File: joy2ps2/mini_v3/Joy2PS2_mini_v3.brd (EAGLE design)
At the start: 25.4 x 47 mm, 8 parts, among them IC1 ATMEGA168PROUND, Q1 BS170

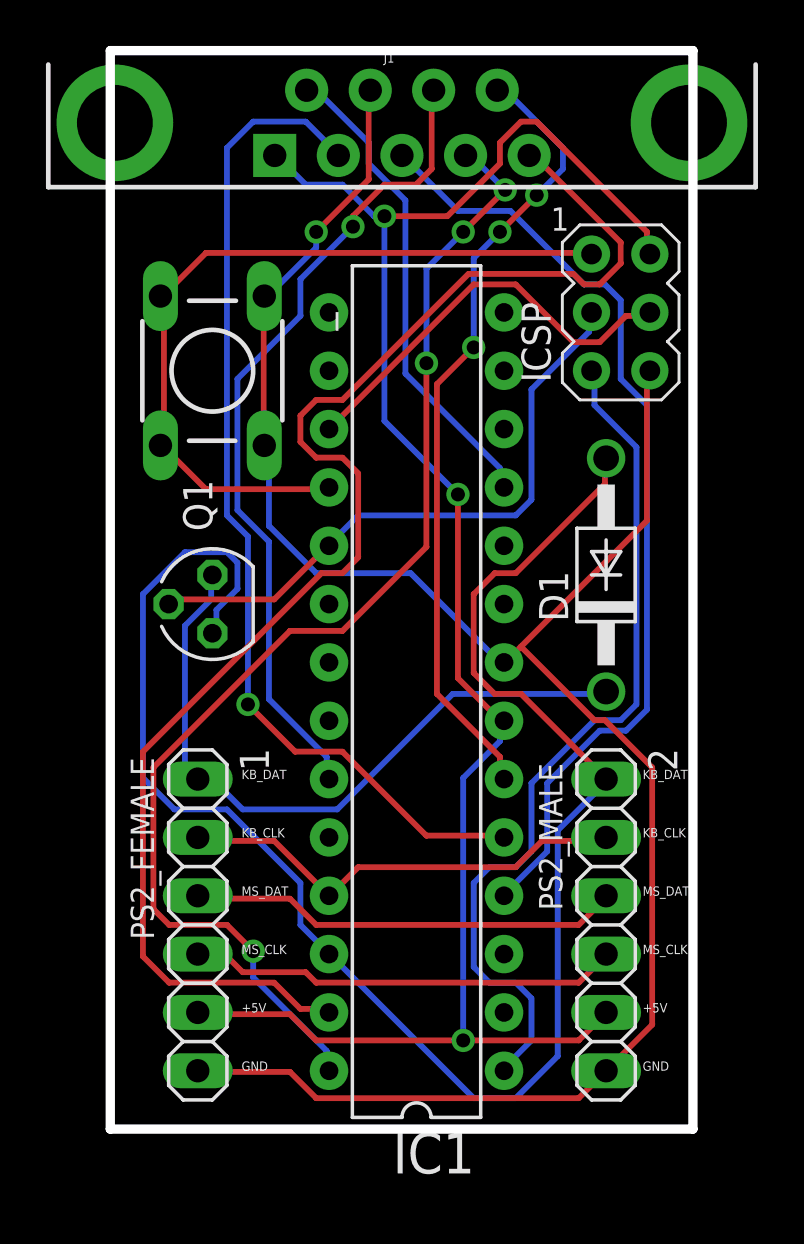
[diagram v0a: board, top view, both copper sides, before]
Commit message: Add files via upload
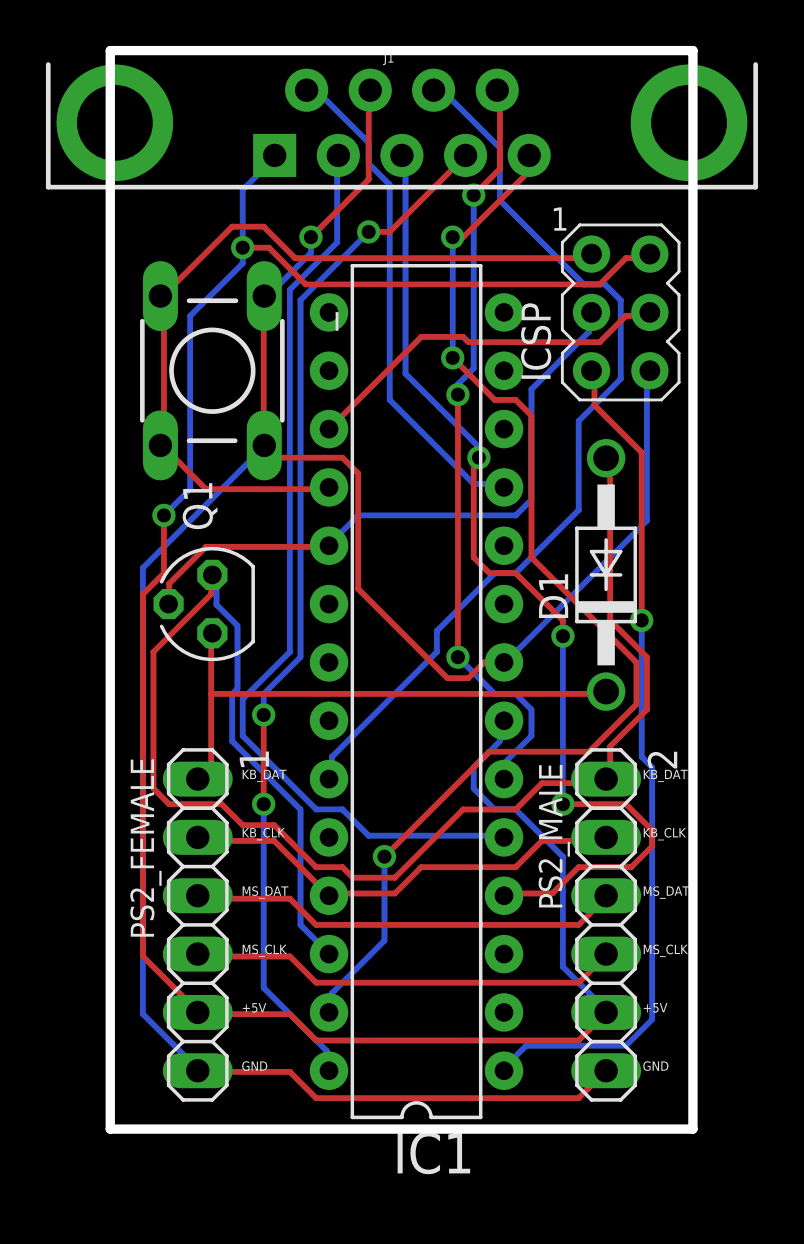
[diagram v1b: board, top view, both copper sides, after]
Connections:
- net KB_DATA: now also Q1.S; no longer Q1.D
- net KB_DATA': now also Q1.D; no longer Q1.S
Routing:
- net +5V: track 80.4 -> 94.8 mm, vias 3 -> 2
- net A4: track 62.4 -> 50.9 mm, vias 0 -> 3
- net GND: track 89.8 -> 99.8 mm
- net A5: track 53.1 -> 45.2 mm, vias 4 -> 3
- net KB_DATA: track 75.4 -> 68.1 mm
- net KB_DATA': track 30.1 -> 23.9 mm
- net A0: track 36.0 -> 40.0 mm, vias 1 -> 0
- net D3: track 44.1 -> 40.2 mm, vias 1 -> 0
- net D2: track 41.8 -> 44.4 mm, vias 0 -> 3
- net D11: track 18.2 -> 16.3 mm
- net D4: track 35.0 -> 33.1 mm
- net D12: track 34.3 -> 35.4 mm
- net RST: track 37.8 -> 36.8 mm, vias 0 -> 1
- net D5: track 21.1 -> 21.8 mm
